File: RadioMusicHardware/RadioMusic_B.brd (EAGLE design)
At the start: 106 x 19.7 mm, 33 parts, among them IC1 TL072P, IC2 TL072P, IC3 7805L, U1 TEENSY_3.1_TW

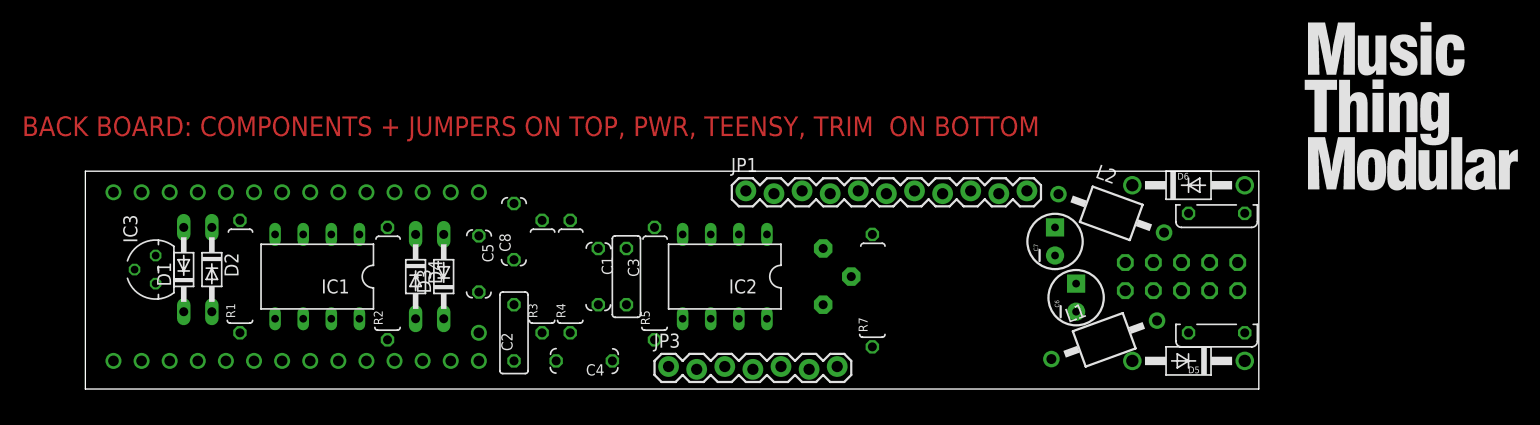
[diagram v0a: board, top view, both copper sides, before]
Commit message: Back board reworking
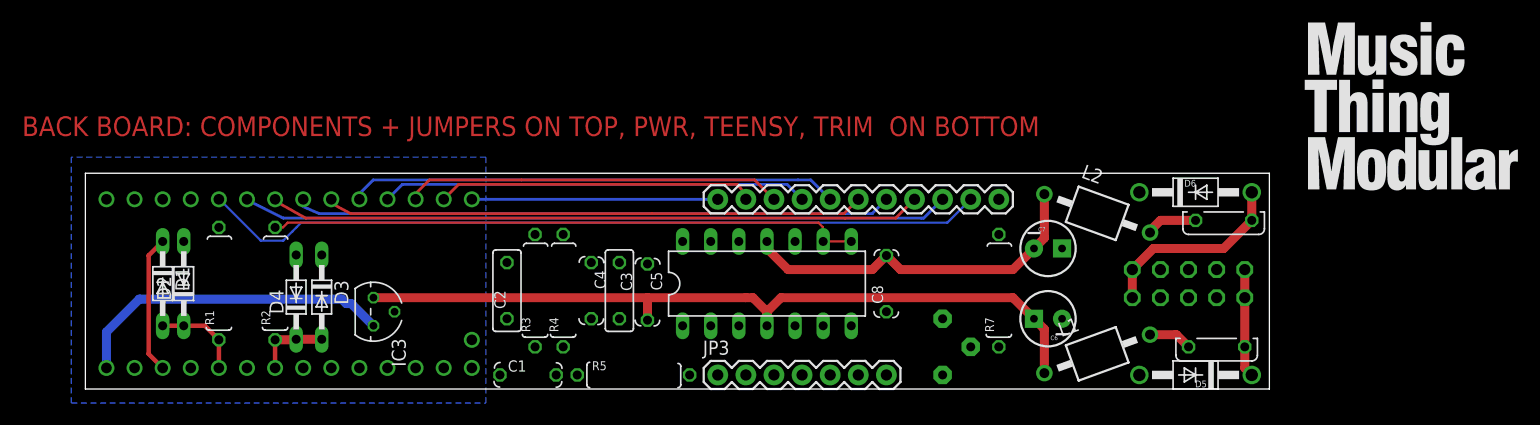
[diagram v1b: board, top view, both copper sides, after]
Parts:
- removed IC1, IC2: TL072P, TomW:DIL08
- removed R6: (no value), bourns:3362P
- added IC4: TL074, linear:DIL14
- added OUTPUT: (no value), bourns:3362P
- D1, D2, D3, D4: value BAT81 -> (none)
- JP1: value M11LOCK -> M11PTH; device SparkFun-Connectors:1X11_LOCK -> SparkFun-Connectors:1X11
- JP3: device SparkFun-Connectors:1X07_LOCK -> SparkFun-Connectors:1X07
- moved C8 34.0 mm to (72.4, 9.53)
- moved JP1 22.9 mm to (82.5, 17.1), turned to 180 degrees
- moved IC3 20.1 mm to (26.0, 6.99), turned to 270 degrees
- moved C5 15.5 mm to (50.8, 8.76)
- moved R7 11.4 mm to (82.5, 8.89)
- moved D3 11.2 mm to (21.4, 8.31), turned to 270 degrees
- moved D4 11.0 mm to (19.1, 8.31), turned to 90 degrees
- moved C1 10.9 mm to (40.0, 1.27), turned to 0 degrees
- moved R2 10.2 mm to (17.1, 9.53)
- moved R5 8.47 mm to (49.5, 1.27), turned to 0 degrees
- moved C4 6.38 mm to (45.7, 8.89), turned to 270 degrees
- moved JP3 4.49 mm to (57.1, 1.27)
- moved C2 3.86 mm to (38.1, 8.89)
- moved C6 3.17 mm to (87.0, 6.35), turned to 180 degrees
- moved D2 2.84 mm to (8.89, 9.53), turned to 90 degrees
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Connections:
- new net N$3: IC4.6, IC4.7, R1.2
- net +12V: now also C5.2, IC4.4; no longer C5.1, IC1.8, IC2.8
- net -12V: now also C8.2, IC4.11; no longer C8.1, IC1.4, IC2.4
- net AUDIO_OUT: now also IC4.1, OUTPUT.2, OUTPUT.3; no longer IC2.1, R6.2, R6.3
- net CHANNEL_CV: now also IC4.5; no longer IC1.3
- net DGND: no longer C5.2, C8.2
- net GND: now also C5.1, C8.1, JP1.1, R7.2; no longer JP1.11, R7.1
- net LED1: now also JP1.2; no longer JP1.1
- net LED2: now also JP1.3; no longer JP1.2
- net LED3: now also JP1.4; no longer JP1.3
- net LED4: now also JP1.5; no longer JP1.4
- net LED_RESET: now also JP1.10; no longer JP1.9
- net MISO: now also JP1.11; no longer JP1.10
- net MOSI: now also JP1.6; no longer JP1.5
- net N$1: now also IC4.8, IC4.9, R2.2; no longer IC1.6, IC1.7, R2.1
- net N$10: now also R3.2; no longer R3.1
- net N$2: now also IC4.12, R4.2; no longer IC2.5, R4.1
- net N$4: now also R3.1, R4.1; no longer R3.2, R4.2
- net N$5: now also C3.1, IC4.13, IC4.14; no longer C3.2, IC2.6, IC2.7
- net N$6: now also C3.2, IC4.3; no longer C3.1, IC2.3
- net N$7: now also IC4.2, OUTPUT.1, R7.1; no longer IC2.2, R6.1, R7.2
- net PIN20/A6: now also R2.1; no longer R2.2
- net PIN22/A8: no longer IC1.1, IC1.2, R1.2
- net RESET_CV: now also JP1.8; no longer JP1.7
- net RESET_SW: now also JP1.7; no longer JP1.6
- net SS: now also JP1.9; no longer JP1.8
- net TIME_CV: now also IC4.10; no longer IC1.5
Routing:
- net +12V: track 0.00 -> 71.4 mm
- net LED1: track 0.00 -> 71.0 mm
- net LED2: track 0.00 -> 64.0 mm
- net LED3: track 0.00 -> 59.0 mm
- net LED4: track 0.00 -> 54.0 mm
- net N$1: track 0.00 -> 53.7 mm
- net MOSI: track 0.00 -> 48.8 mm
- net RESET_SW: track 0.00 -> 44.3 mm
- net RESET_CV: track 0.00 -> 38.6 mm
- net SS: track 0.00 -> 34.1 mm
- net -12V: track 0.00 -> 32.7 mm
- net +5V: track 0.00 -> 29.6 mm
- net LED_RESET: track 0.00 -> 28.7 mm
- net MISO: track 0.00 -> 22.2 mm
- net -12V_INLET: track 0.00 -> 17.7 mm
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- added copper zone on layer 16, net DGND
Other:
- board size 106 x 19.7 mm -> 107 x 19.5 mm
